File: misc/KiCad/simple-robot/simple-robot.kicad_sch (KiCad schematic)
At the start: 54 parts, among them M3 Motor_Servo, U1 Pico2

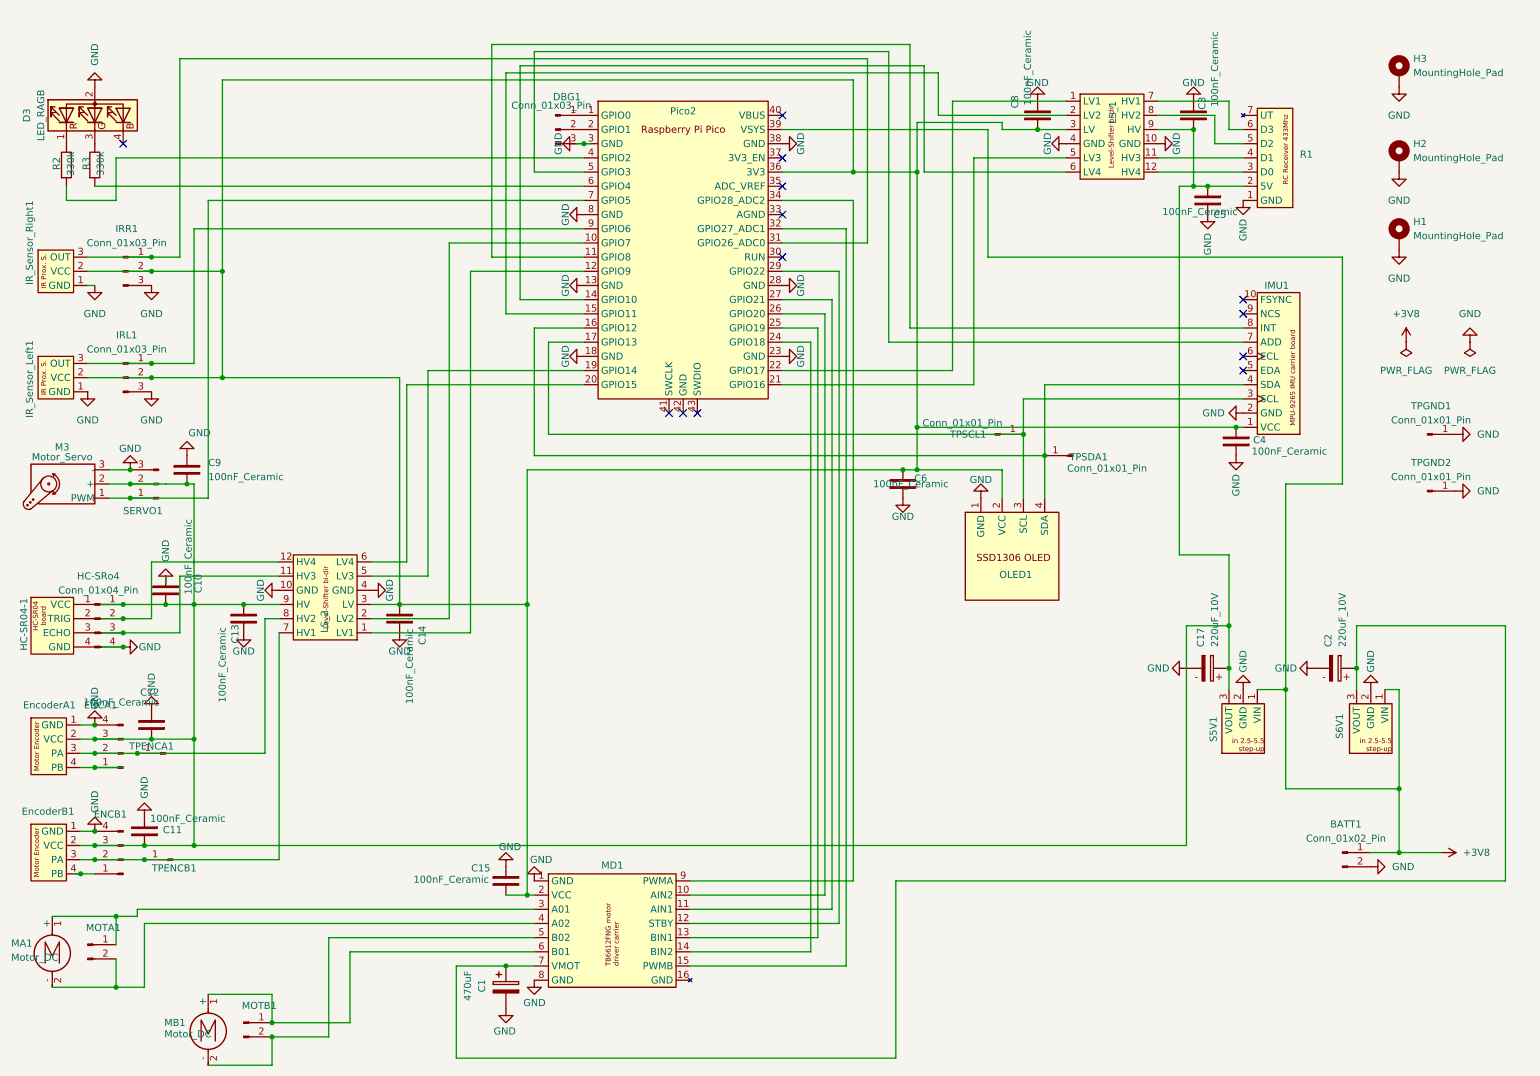
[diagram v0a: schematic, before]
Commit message: Upgrade KiCad project and schematic files
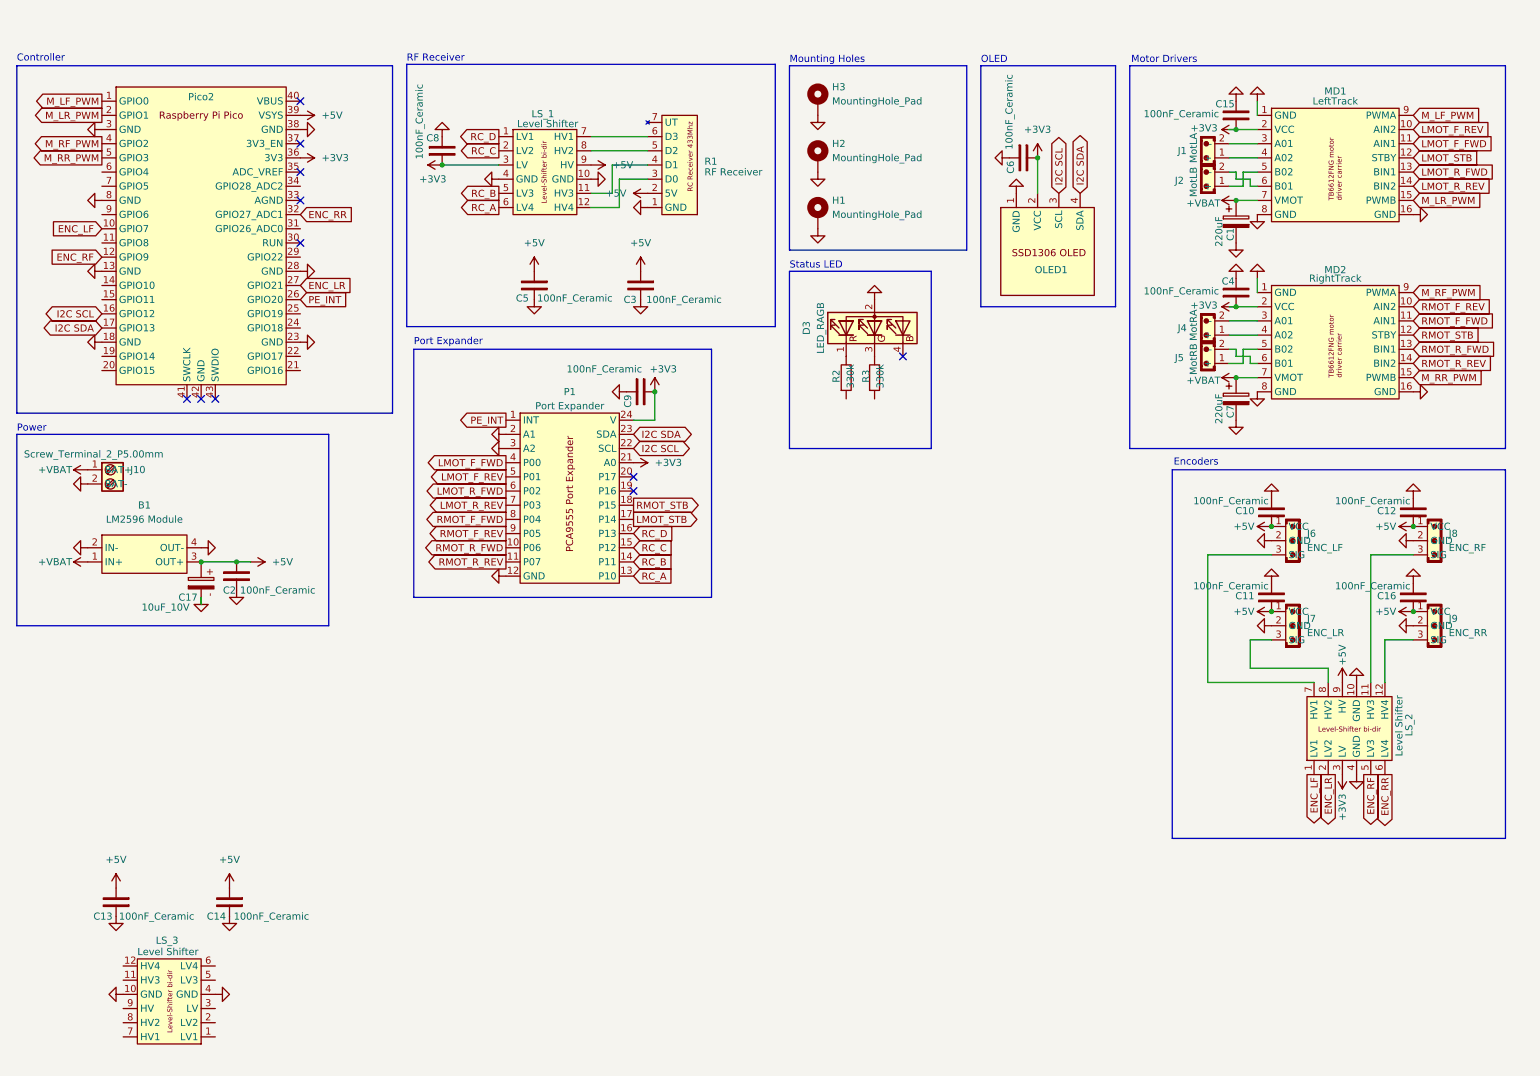
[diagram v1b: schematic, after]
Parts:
- removed BATT1: Conn_01x02_Pin, Connector_PinHeader_2.54mm:PinHeader_1x02_P2.54mm_Vertical, symbol Connector:Conn_01x02_Pin
- removed C2: 220uF_10V, Capacitor_THT:CP_Radial_D6.3mm_P2.50mm, symbol PCM_SL_Capacitors:220uF_10V
- removed DBG1, IRL1, IRR1, SERVO1: Conn_01x03_Pin, Connector_PinHeader_2.54mm:PinHeader_1x03_P2.54mm_Vertical, symbol Connector:Conn_01x03_Pin
- removed ENCA1, ENCB1, HC-SRo4: Conn_01x04_Pin, Connector_PinHeader_2.54mm:PinHeader_1x04_P2.54mm_Vertical, symbol Connector:Conn_01x04_Pin
- removed EncoderA1, EncoderB1: ~, symbol common-hobby-things:Hall-effect_encoder
- removed HC-SR04-1: ~, symbol common-hobby-things:HC-SR04
- removed IMU1: ~, common-hobby-things:MPU 9265 IMU carrier board, symbol common-hobby-things:GY-9250_9-Axis
- removed IR_Sensor_Left1, IR_Sensor_Right1: ~, symbol common-hobby-things:IR_Proximity_Sensor
- removed M3: Motor_Servo, symbol Motor:Motor_Servo
- removed MA1, MB1: Motor_DC, symbol Motor:Motor_DC
- removed MOTA1, MOTB1: ~, Connector_PinHeader_2.54mm:PinHeader_1x02_P2.54mm_Vertical, symbol Connector:Conn_01x02_Pin
- removed S5V1: ~, common-hobby-things:Pololu step-up converter 2.5-5.5V in 5V out, symbol common-hobby-things:step-up-converter_5V
- removed S6V1: ~, common-hobby-things:Pololu step-up converter 2.5-5.5V in 6V out, symbol common-hobby-things:step-up-converter_6V
- removed TPENCA1, TPENCB1, TPGND1, TPGND2, TPSCL1, TPSDA1: Conn_01x01_Pin, Connector_PinHeader_2.54mm:PinHeader_1x01_P2.54mm_Vertical, symbol Connector:Conn_01x01_Pin
- added B1: LM2596 Module, symbol common-hobby-things:LM2596_Module
- added C16, C2: 100nF_Ceramic, Capacitor_THT:C_Disc_D5.0mm_W2.5mm_P2.50mm, symbol PCM_SL_Capacitors:100nF_Ceramic
- added C7: 220uF, Capacitor_THT:CP_Radial_D6.3mm_P2.50mm, symbol Device:C_Polarized
- added J1: MotLA, Connector_JST:JST_PH_B2B-PH-K_1x02_P2.00mm_Vertical, symbol PCM_SL_Connectors:JST_02
- added J10: Screw_Terminal_2_P5.00mm, TerminalBlock_Phoenix:TerminalBlock_Phoenix_PT-1,5-2-5.0-H_1x02_P5.00mm_Horizontal, symbol PCM_SL_Screw_Terminal:Screw_Terminal_2_P5.00mm
- added J2: MotLB, Connector_JST:JST_PH_B2B-PH-K_1x02_P2.00mm_Vertical, symbol PCM_SL_Connectors:JST_02
- added J4: MotRA, Connector_JST:JST_PH_B2B-PH-K_1x02_P2.00mm_Vertical, symbol PCM_SL_Connectors:JST_02
- added J5: MotRB, Connector_JST:JST_PH_B2B-PH-K_1x02_P2.00mm_Vertical, symbol PCM_SL_Connectors:JST_02
- added J6: ENC_LF, Connector_JST:JST_PH_B3B-PH-K_1x03_P2.00mm_Vertical, symbol PCM_SL_Connectors:JST_03
- added J7: ENC_LR, Connector_JST:JST_PH_B3B-PH-K_1x03_P2.00mm_Vertical, symbol PCM_SL_Connectors:JST_03
- added J8: ENC_RF, Connector_JST:JST_PH_B3B-PH-K_1x03_P2.00mm_Vertical, symbol PCM_SL_Connectors:JST_03
- added J9: ENC_RR, Connector_JST:JST_PH_B3B-PH-K_1x03_P2.00mm_Vertical, symbol PCM_SL_Connectors:JST_03
- added LS_3: Level Shifter, common-hobby-things:Level shifter 4 bi-dir, symbol common-hobby-things:level-shifter
- added MD2: RightTrack, common-hobby-things:TB6612FNG motor driver carrier, symbol common-hobby-things:TB6612FNG motor driver carrier
- added P1: Port Expander, symbol common-hobby-things:PCA9555
- C1: value 470uF -> 220uF
- C17: value 220uF_10V -> 10uF_10V
- LS_1, LS_2: value ~ -> Level Shifter
- MD1: value ~ -> LeftTrack
- R1: value ~ -> RF Receiver
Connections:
- net +3V8 is gone; now on net +5V: U1.39 (VSYS)
- net GND: now also C11.2, C12.2, C9.1, MD1.16 (GND), B1.2 (IN-), B1.4 (OUT-), C16.2, C2.1, C7.2, J10.2 (BAT-), J6.2 (GND), J7.2 (GND), J8.2 (GND), J9.2 (GND), LS_3.10 (GND), LS_3.4 (GND), MD2.1 (GND), MD2.16 (GND), MD2.8 (GND), P1.12 (GND), P1.2 (A1), P1.3 (A2); no longer C11.1, C12.1, C9.2
- net at LS_2.7 (HV1): now also J6.3 (SIG)
- net +3V3: now reaches C15.1, C4.1, C6.2, C8.1, LS_1.3 (LV), LS_2.3 (LV), MD1.2 (VCC), OLED1.2 (VCC), U1.36 (3V3)
- net +3V3: now also C9.2, MD2.2 (VCC), P1.21 (A0), P1.24 (V); no longer C14.1
- net +5V: now reaches C10.1, C13.1, C17.1, C3.1, C5.1, LS_1.9 (HV), LS_2.9 (HV), R1.2 (5V)
- net +5V: now also C11.1, C12.1, C14.1, B1.3 (OUT+), C16.1, C2.2, J6.1 (VCC), J7.1 (VCC), J8.1 (VCC), J9.1 (VCC); no longer C11.2, C12.2, C9.1
- net at R2.1: no longer U1.4 (GPIO2)
- net I2C SCL: now reaches U1.16 (GPIO12)
- net I2C SCL: now also OLED1.3 (SCL), P1.22 (SCL); no longer OLED1.4 (SDA)
- net +VBAT: now reaches C1.1, MD1.7 (VMOT)
- net +VBAT: now also B1.1 (IN+), C7.1, J10.1 (BAT+), MD2.7 (VMOT)
- net at MD1.3 (A01): now also J1.2 (-)
- net at MD1.4 (A02): now also J1.1 (+)
- net M_LF_PWM: now reaches U1.1 (GPIO0)
- net M_LF_PWM: now also MD1.9 (PWMA)
- net M_LR_PWM: now reaches U1.2 (GPIO1)
- net M_LR_PWM: now also MD1.15 (PWMB)
- net at R3.1: no longer U1.6 (GPIO4)
- net LMOT_F_REV: now reaches MD1.10 (AIN2)
- net LMOT_F_REV: now also P1.5 (P01); no longer U1.26 (GPIO20)
- net ENC_LR: now reaches U1.27 (GPIO21)
- net ENC_LR: now also LS_2.2 (LV2); no longer MD1.11 (AIN1)
- net at U1.29 (GPIO22): no longer MD1.12 (STBY)
- net at U1.25 (GPIO19): no longer MD1.13 (BIN1)
- net at U1.24 (GPIO18): no longer MD1.14 (BIN2)
- net ENC_RR: now reaches U1.32 (GPIO27_ADC1)
- net ENC_RR: now also LS_2.6 (LV4); no longer MD1.15 (PWMB)
- net at MD1.5 (B02): now also J2.1 (+)
- net at MD1.6 (B01): now also J2.2 (-)
- net at U1.34 (GPIO28_ADC2): no longer MD1.9 (PWMA)
- net at LS_2.8 (HV2): now also J7.3 (SIG)
- net ENC_LF: now reaches LS_2.1 (LV1)
- net ENC_LF: now also U1.10 (GPIO7); no longer U1.12 (GPIO9)
- net at LS_2.11 (HV3): now also J8.3 (SIG)
- net at LS_2.12 (HV4): now also J9.3 (SIG)
- net at U1.19 (GPIO14): no longer LS_2.5 (LV3)
- net at U1.20 (GPIO15): no longer LS_2.6 (LV4)
- net I2C SDA: now reaches U1.17 (GPIO13)
- net I2C SDA: now also OLED1.4 (SDA), P1.23 (SDA); no longer OLED1.3 (SCL)
- net at U1.22 (GPIO17): no longer LS_1.1 (LV1)
- net at U1.15 (GPIO11): no longer LS_1.2 (LV2)
- net at U1.21 (GPIO16): no longer LS_1.5 (LV3)
- net at U1.14 (GPIO10): no longer LS_1.6 (LV4)
- net M_RR_PWM: now reaches U1.5 (GPIO3)
- net M_RR_PWM: now also MD2.15 (PWMB)
- new net: J4.1 (+), MD2.4 (A02)
- new net: J4.2 (-), MD2.3 (A01)
- new net: J5.1 (+), MD2.5 (B02)
- new net: J5.2 (-), MD2.6 (B01)
- new net ENC_RF: LS_2.5 (LV3), U1.12 (GPIO9)
- new net LMOT_F_FWD: MD1.11 (AIN1), P1.4 (P00)
- new net LMOT_R_FWD: MD1.13 (BIN1), P1.6 (P02)
- new net LMOT_R_REV: MD1.14 (BIN2), P1.7 (P03)
- new net LMOT_STB: MD1.12 (STBY), P1.17 (P14)
- new net M_RF_PWM: MD2.9 (PWMA), U1.4 (GPIO2)
- new net PE_INT: P1.1 (INT), U1.26 (GPIO20)
- new net RC_A: LS_1.6 (LV4), P1.13 (P10)
- new net RC_B: LS_1.5 (LV3), P1.14 (P11)
- new net RC_C: LS_1.2 (LV2), P1.15 (P12)
- new net RC_D: LS_1.1 (LV1), P1.16 (P13)
- new net RMOT_F_FWD: MD2.11 (AIN1), P1.8 (P04)
- new net RMOT_F_REV: MD2.10 (AIN2), P1.9 (P05)
- new net RMOT_R_FWD: MD2.13 (BIN1), P1.10 (P06)
- new net RMOT_R_REV: MD2.14 (BIN2), P1.11 (P07)
- new net RMOT_STB: MD2.12 (STBY), P1.18 (P15)
- no-connect marks 13 -> 11
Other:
- note added: "Controller"
- note added: "Encoders"
- note added: "Motor Drivers"
- note added: "Mounting Holes"
- note added: "OLED"
- note added: "Port Expander"
- note added: "Power"
- note added: "RF Receiver"
- note added: "Status LED"
- moved on the sheet: C1, C13, C14, C15, C17, C3, C5, C6, C8, D3, H1, H2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
